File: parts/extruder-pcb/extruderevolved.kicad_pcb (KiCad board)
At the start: 2 copper layers, 68 x 57 mm, 8 parts, among them CN1 B-3102R24P-A000, CN2 HC-1.25-2PWT, CN3 HC-1.25-3PWT, CN4 HC-1.25-4PWT, CN5 HC-1.25-5PWT, CN6 X2011WRS-02A-9TSN, CN7 HC-1.25-2PWT, CN8 HC-1.25-2PWT

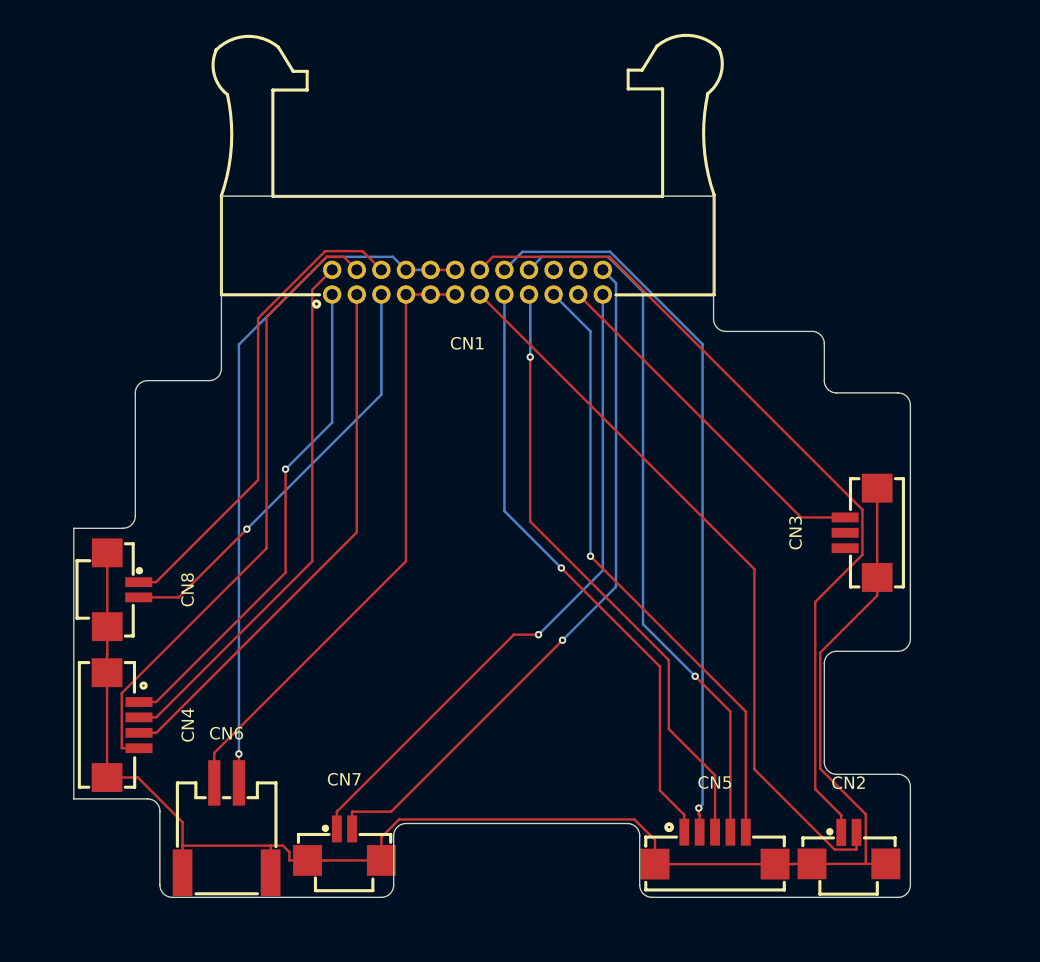
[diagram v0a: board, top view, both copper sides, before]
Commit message: Add files via upload
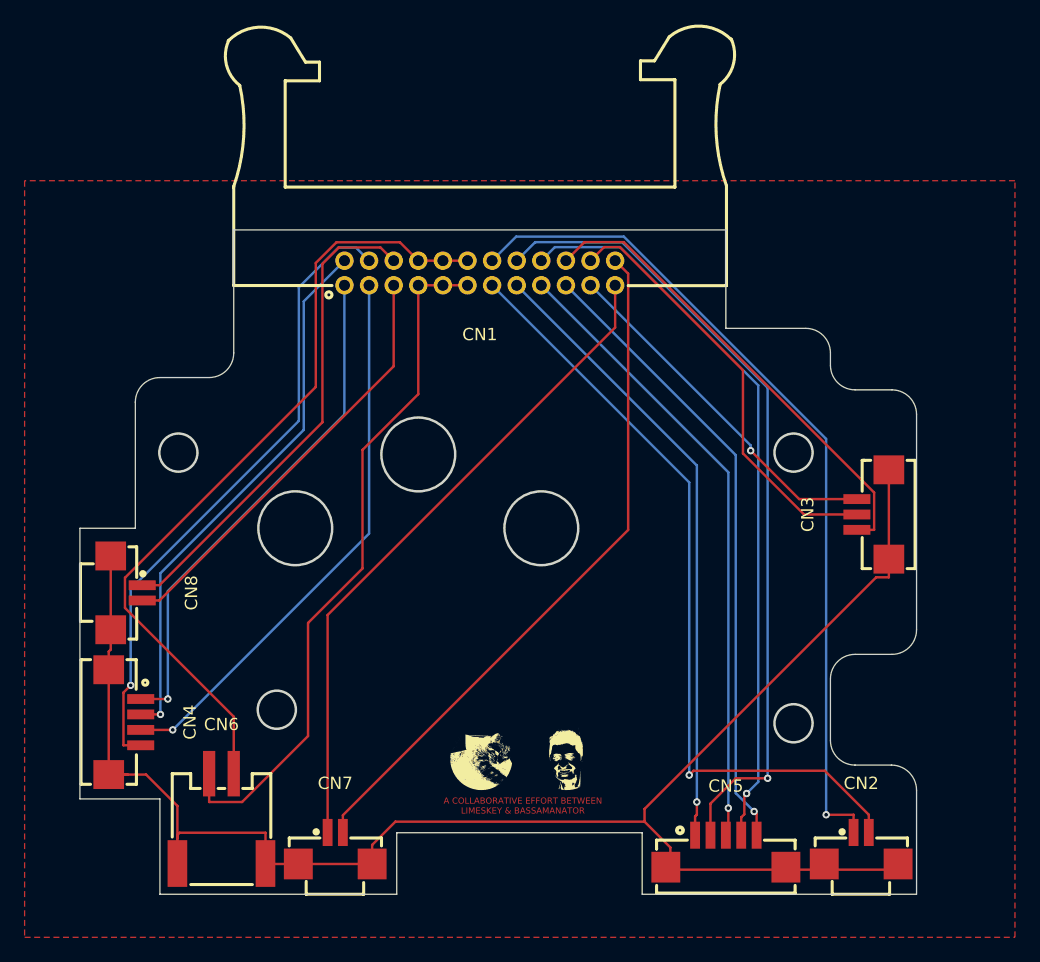
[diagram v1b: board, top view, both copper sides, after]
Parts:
- added G***: LOGO, Images:limskeyyy, F.Cu at (152.0, 104.8)
- added basamator: LOGO, Images:basa, F.Cu at (159.5, 104.1)
- moved CN3 1.77 mm to (183.9, 84.9)
- moved CN1 1.25 mm to (152.0, 65.2)
- moved CN2 1.00 mm to (183.0, 112.0)
- moved CN5 0.91 mm to (172.0, 112.2)
- moved CN6 0.86 mm to (131.0, 109.6)
- moved CN7 0.80 mm to (140.2, 112.0)
- moved CN8 0.38 mm to (123.3, 91.2)
- moved CN4 0.28 mm to (123.1, 101.8)
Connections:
- net Empty "DET" #1 renamed Empty DET #1
- net Empty "DET" #2 renamed Empty DET #2
- net Empty "DET" #3 renamed Empty DET #3
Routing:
- net Empty DET #1: track 0.00 -> 38.5 mm
- net Empty DET #2: track 0.00 -> 35.1 mm
- net Heater-: track 56.6 -> 65.4 mm, vias 1 -> 0
- net GND: track 129.4 -> 136.8 mm
- net Heater+: track 50.2 -> 56.8 mm
- net Probe #2: track 59.6 -> 65.9 mm
- net Part Cooling Fan-: track 60.2 -> 64.1 mm, vias 0 -> 1
- net Probe #4: track 57.7 -> 60.1 mm
- net E Motor #3: track 43.8 -> 45.4 mm, vias 0 -> 1
- net E Motor #1: track 40.4 -> 41.8 mm
- net Probe #3: track 50.0 -> 51.3 mm
- net Probe #1: track 49.8 -> 51.0 mm
- net Probe #5: track 50.2 -> 51.3 mm
- net E Motor #2: track 43.7 -> 44.7 mm, vias 0 -> 1
- net E Motor #4: track 51.1 -> 52.0 mm, vias 0 -> 1
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- added copper zone on F.Cu, net (none)
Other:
- board size 68 x 57 mm -> 68 x 54 mm
- board text added: "A COLLABORATIVE EFFORT BETWEEN LIMESKEY & BASSAMANATOR"
